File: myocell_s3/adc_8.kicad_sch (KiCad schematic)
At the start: 45 parts, among them U1 OPA340NA, U2 ADS1298xPAG, U3 OPA340NA

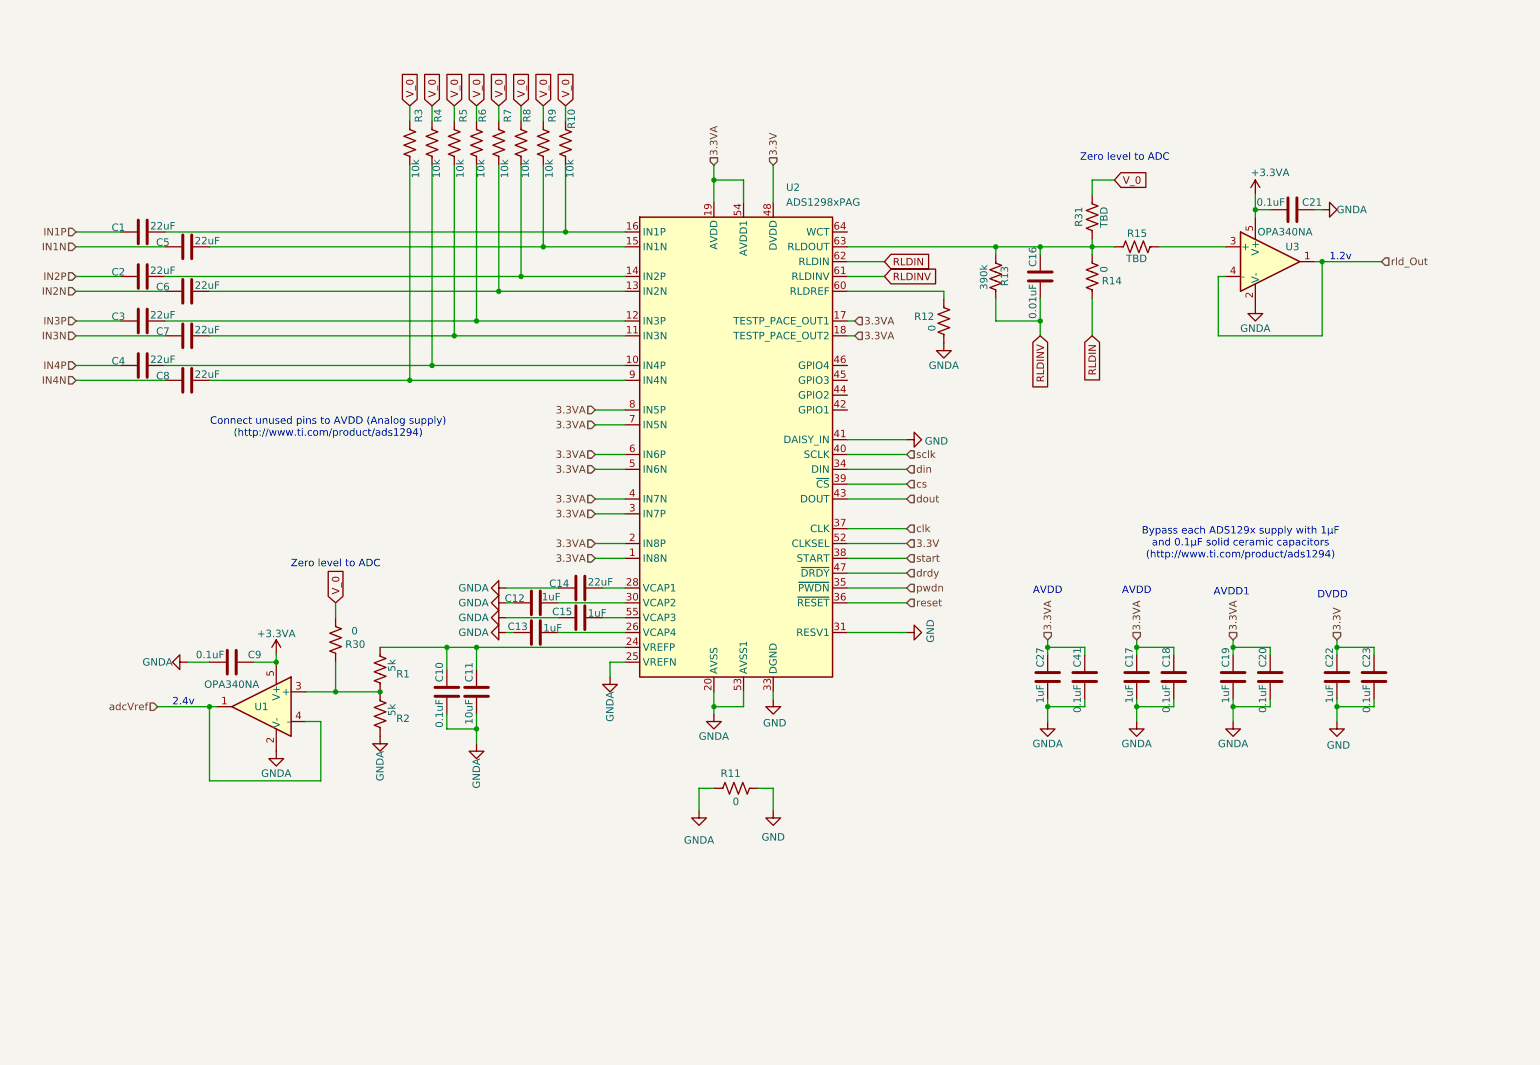
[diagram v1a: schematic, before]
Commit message: working on schematic
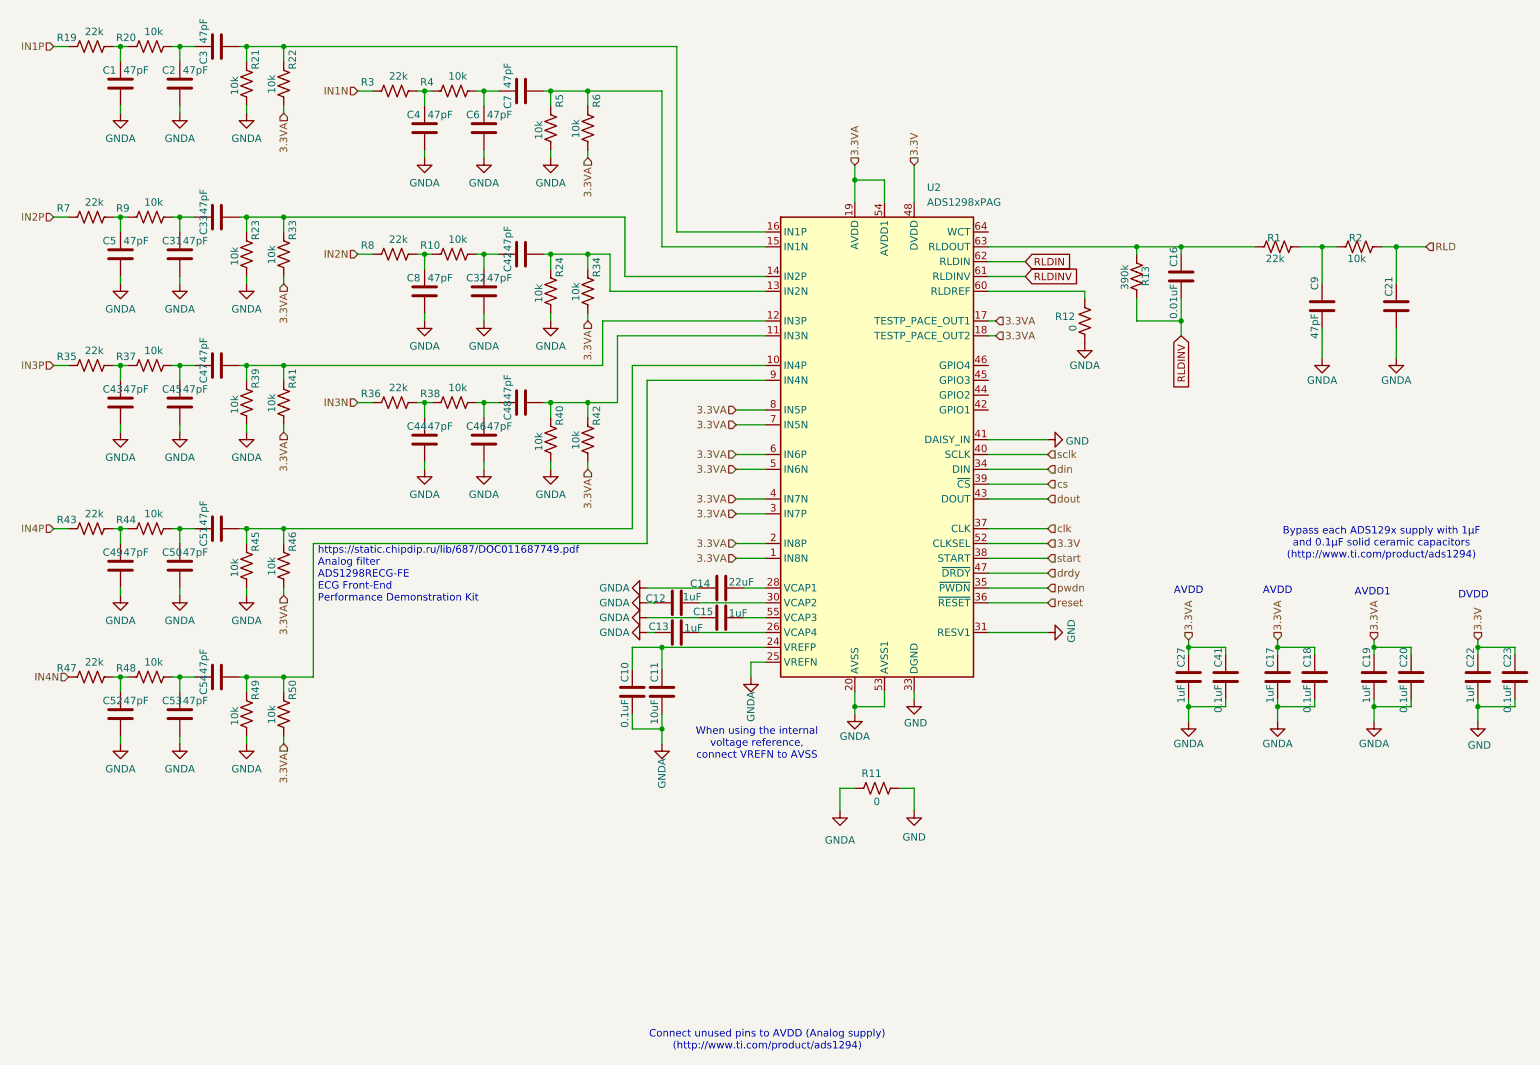
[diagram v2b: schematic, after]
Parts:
- removed R14, R30: 0, Resistor_SMD:R_0805_2012Metric_Pad1.20x1.40mm_HandSolder, symbol Device:R_US
- removed R15, R31: TBD, Resistor_SMD:R_0805_2012Metric_Pad1.20x1.40mm_HandSolder, symbol Device:R_US
- removed U1, U3: OPA340NA, Package_TO_SOT_SMD:SOT-23-5, symbol Amplifier_Operational:OPA340NA
- added C31, C32, C33, C42, C43, C44, C45, C46, C47, C48, C49, C50, C51, C52, C53, C54: 47pF, Capacitor_SMD:C_0805_2012Metric_Pad1.18x1.45mm_HandSolder, symbol Device:C
- added R19, R35, R36, R43, R47: 22k, Resistor_SMD:R_0805_2012Metric_Pad1.20x1.40mm_HandSolder, symbol Device:R_US
- added R20, R21, R22, R23, R24, R33, R34, R37, R38, R39, R40, R41, R42, R44, R45, R46, R48, R49, R50: 10k, Resistor_SMD:R_0805_2012Metric_Pad1.20x1.40mm_HandSolder, symbol Device:R_US
- C1, C2, C3, C4, C5, C6, C7, C8: value 22uF -> 47pF
- C21: value 0.1uF -> ~
- C9: value 0.1uF -> 47pF
- R1: value 5k -> 22k
- R2: value 5k -> 10k
- R3, R7, R8: value 10k -> 22k
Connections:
- net 3.3VA: now also R6.2, R22.2, R33.2, R34.2, R41.2, R42.2, R46.2, R50.2
- net GNDA: now also C1.2, C2.2, C21.1, C4.2, C5.2, C6.2, C8.2, R5.2, C31.2, C32.2, C43.2, C44.2, C45.2, C46.2, C49.2, C50.2, C52.2, C53.2, R21.2, R23.2, R24.2, R39.2, R40.2, R45.2, R49.2; no longer C21.2, R2.2
- net IN1N: now also R3.1; no longer C5.2
- net IN1P: now also R19.1; no longer C1.2
- net IN2N: now also R8.1; no longer C6.2
- net IN2P: now also R7.1; no longer C2.2
- net IN3N: now also R36.1; no longer C7.2
- net IN3P: now also R35.1; no longer C3.2
- net IN4N: now also R47.1; no longer C8.2
- net IN4P: now also R43.1; no longer C4.2
- net at C16.2, R13.1, U2.63 (RLDOUT): now also R1.1
- net at C10.2, C11.2, U2.24 (VREFP): no longer R1.1
- net at R1.2, R2.1: now also C9.2
- removed net +3.3VA: C21.1, C9.2
- removed net V_0: R10.1, R3.1, R4.1, R5.1, R6.1, R7.1, R8.1, R9.1
- new net: C32.1, C42.1, R10.2
- new net: C2.1, C3.1, R20.2
- new net: C3.2, R21.1, R22.1, U2.16 (IN1P)
- new net: C31.1, C33.1, R9.2
- new net: C7.2, R5.1, R6.1, U2.15 (IN1N)
- new net: C53.1, C54.1, R48.2
- new net: C54.2, R49.1, R50.1, U2.9 (IN4N)
- new net: C42.2, R24.1, R34.1, U2.13 (IN2N)
- new net: C44.1, R36.2, R38.1
- new net: C52.1, R47.2, R48.1
- new net: C51.2, R45.1, R46.1, U2.10 (IN4P)
- new net: C48.2, R40.1, R42.1, U2.11 (IN3N)
- new net: C47.2, R39.1, R41.1, U2.12 (IN3P)
- new net: C33.2, R23.1, R33.1, U2.14 (IN2P)
- new net: C8.1, R10.1, R8.2
- new net: C6.1, C7.1, R4.2
- new net: C1.1, R19.2, R20.1
- new net: C45.1, C47.1, R37.2
- new net: C43.1, R35.2, R37.1
- new net: C4.1, R3.2, R4.1
- new net: C50.1, C51.1, R44.2
- new net: C49.1, R43.2, R44.1
- new net: C5.1, R7.2, R9.1
- new net: C46.1, C48.1, R38.2
- new net RLD: C21.2, R2.2
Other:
- note added: "When using the internal voltage reference, connect VREFN to AVSS"
- note added: "https://static.chipdip.ru/lib/687/DOC011687749.pdf Analog filter ADS1298RECG-FE ECG Front-End Performance Demonstration Kit"
- note removed: "1.2v"
- note removed: "2.4v"
- note removed: "Zero level to ADC"
- moved on the sheet: C1, C10, C11, C12, C13, C14, C15, C16, C17, C18, C19, C20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
